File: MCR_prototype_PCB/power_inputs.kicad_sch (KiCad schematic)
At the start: 11 parts, among them J1 Conn_01x20_Pin, U20 LM2596T-5, U21 LM2596T-3.3

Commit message: Add files via upload
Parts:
- C5, C7: footprint (none) -> Capacitor_THT:CP_Radial_D10.0mm_P5.00mm; KiLib_Generator (none) -> capacitor/THT/other
- C6, C8: footprint (none) -> Capacitor_THT:CP_Radial_D8.0mm_P3.50mm; KiLib_Generator (none) -> capacitor/THT/other
- D1, D2: KiLib_Generator (none) -> diode/THT
- J1: footprint (none) -> Connector_PinHeader_2.54mm:PinHeader_1x20_P2.54mm_Horizontal; KiLib_Generator (none) -> connector/pin_header_socket
- L1, L2: footprint (none) -> Inductor_SMD:L_Bourns_SRR1260
- U20, U21: KiLib_Generator (none) -> package/TO_SOT/THT
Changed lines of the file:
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@@
+			)
+		)
+		(property "KiLib_Generator" "diode/THT"
+			(at 125.73 77.47 0)
+			(hide yes)
+			(show_name no)
+			(do_not_autoplace no)
+			(effects
+				(font
+					(size 1.27 1.27)
+				)
 			)
 		)
@@
 			)
 		)
-		(property "Footprint" ""
+		(property "Footprint" "Inductor_SMD:L_Bourns_SRR1260"
 			(at 132.08 73.66 0)
 			(hide yes)
@@
 			)
 		)
+		(property "KiLib_Generator" "diode/THT"
+			(at 124.46 39.37 0)
+			(hide yes)
+			(show_name no)
+			(do_not_autoplace no)
+			(effects
+				(font
+					(size 1.27 1.27)
+				)
+			)
+		)
 		(pin "1"
 		)
@@
 			)
 		)
-		(property "Footprint" ""
+		(property "Footprint" "Capacitor_THT:CP_Radial_D10.0mm_P5.00mm"
 			(at 82.55 71.12 0)
 			(hide yes)
@@
 		)
 		(property "Description" "capacitor, small US symbol"
+			(at 82.55 71.12 0)
+			(hide yes)
+			(show_name no)
+			(do_not_autoplace no)
+			(effects
+				(font
+					(size 1.27 1.27)
+				)
+			)
+		)
+		(property "KiLib_Generator" "capacitor/THT/other"
 			(at 82.55 71.12 0)
 			(hide yes)
@@
 			)
 		)
-		(property "Footprint" ""
+		(property "Footprint" "Inductor_SMD:L_Bourns_SRR1260"
 			(at 130.81 35.56 0)
 			(hide yes)
@@
 			)
 		)
+		(property "KiLib_Generator" "package/TO_SOT/THT"
+			(at 104.14 33.02 0)
+			(hide yes)
+			(show_name no)
+			(do_not_autoplace no)
+			(effects
+				(font
+					(size 1.27 1.27)
+				)
+			)
+		)
 		(pin "5"
 		)
@@
 			)
 		)
-		(property "Footprint" ""
+		(property "Footprint" "Capacitor_THT:CP_Radial_D10.0mm_P5.00mm"
 			(at 82.55 33.02 0)
 			(hide yes)
@@
 		)
 		(property "Description" "capacitor, small US symbol"
+			(at 82.55 33.02 0)
+			(hide yes)
+			(show_name no)
+			(do_not_autoplace no)
+			(effects
+				(font
+					(size 1.27 1.27)
+				)
+			)
+		)
+		(property "KiLib_Generator" "capacitor/THT/other"
 			(at 82.55 33.02 0)
 			(hide yes)
@@
 			)
 		)
+		(property "KiLib_Generator" "package/TO_SOT/THT"
+			(at 104.14 71.12 0)
+			(hide yes)
+			(show_name no)
+			(do_not_autoplace no)
+			(effects
+				(font
+					(size 1.27 1.27)
+				)
+			)
+		)
 		(pin "1"
 		)
@@
 			)
 		)
-		(property "Footprint" ""
+		(property "Footprint" "Connector_PinHeader_2.54mm:PinHeader_1x20_P2.54mm_Horizontal"
 			(at 34.29 50.8 0)
 			(hide yes)
@@
 		)
 		(property "Description" "Generic connector, single row, 01x20, script generated"
+			(at 34.29 50.8 0)
+			(hide yes)
+			(show_name no)
+			(do_not_autoplace no)
+			(effects
+				(font
+					(size 1.27 1.27)
+				)
+			)
+		)
+		(property "KiLib_Generator" "connector/pin_header_socket"
 			(at 34.29 50.8 0)
 			(hide yes)
@@
 			)
 		)
-		(property "Footprint" ""
+		(property "Footprint" "Capacitor_THT:CP_Radial_D8.0mm_P3.50mm"
 			(at 137.16 38.1 0)
 			(hide yes)
@@
 		)
 		(property "Description" "capacitor, small US symbol"
+			(at 137.16 38.1 0)
+			(hide yes)
+			(show_name no)
+			(do_not_autoplace no)
+			(effects
+				(font
+					(size 1.27 1.27)
+				)
+			)
+		)
+		(property "KiLib_Generator" "capacitor/THT/other"
 			(at 137.16 38.1 0)
 			(hide yes)
@@
 			)
 		)
-		(property "Footprint" ""
+		(property "Footprint" "Capacitor_THT:CP_Radial_D8.0mm_P3.50mm"
 			(at 138.43 76.2 0)
 			(hide yes)
@@
 			(at 138.43 76.2 0)
 			(hide yes)
+			(show_name no)
+			(do_not_autoplace no)
+			(effects
+				(font
+					(size 1.27 1.27)
+				)
+			)
+		)
+		(property "KiLib_Generator" "capacitor/THT/other"
+			(at 138.43 76.2 0)
+			(hide yes)

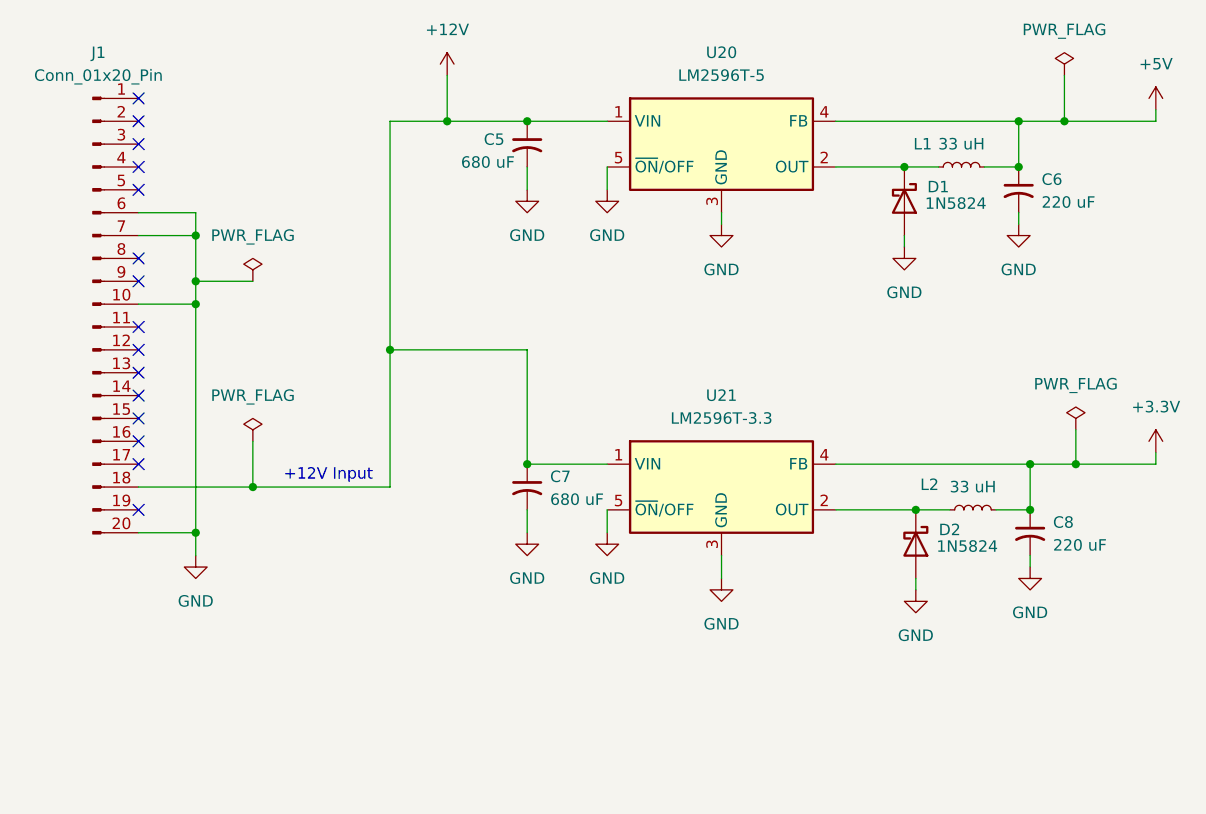
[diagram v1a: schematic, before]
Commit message: Updated 8/22/26
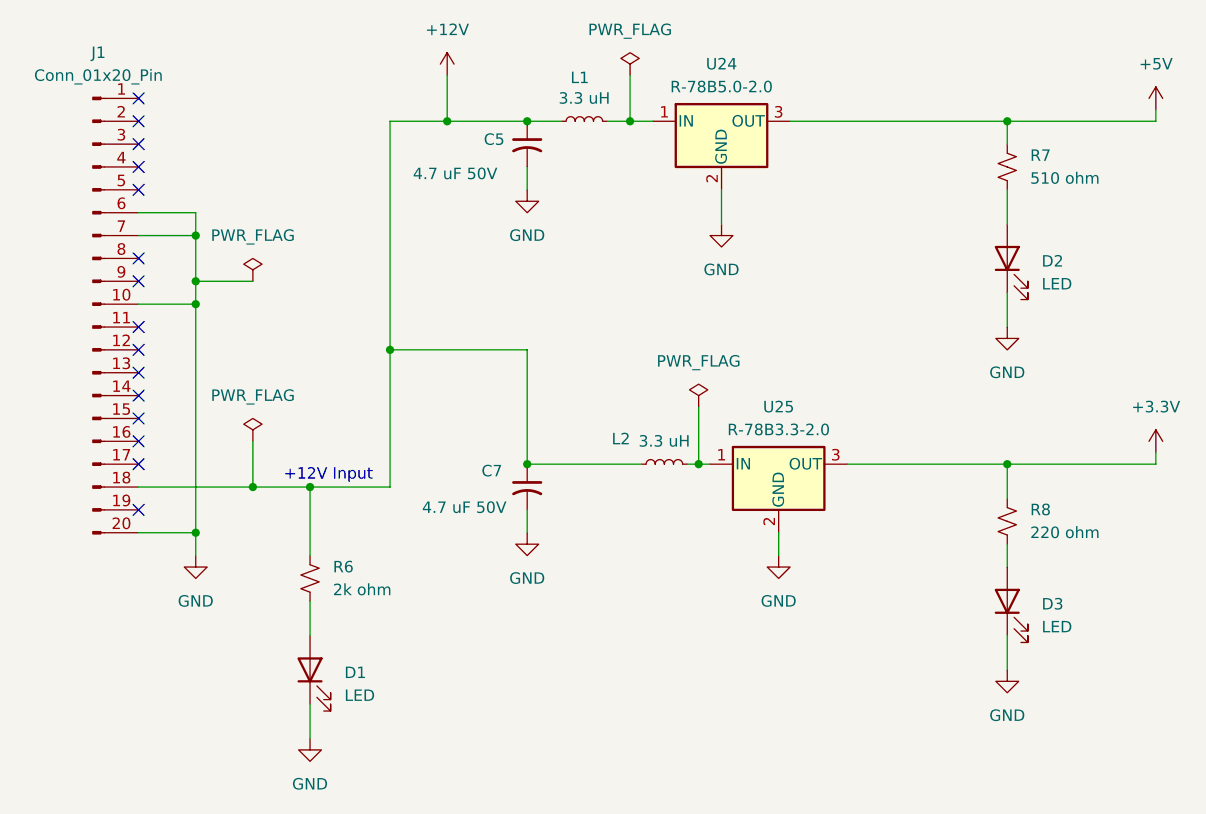
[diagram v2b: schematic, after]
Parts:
- removed C6, C8: 220 uF, Capacitor_THT:CP_Radial_D8.0mm_P3.50mm, symbol Device:C_Small_US
- removed D1, D2: 1N5824, Diode_THT:D_DO-201AD_P15.24mm_Horizontal, symbol Diode:1N5822
- removed U20: LM2596T-5, Package_TO_SOT_THT:TO-220-5_P3.4x3.7mm_StaggerOdd_Lead3.8mm_Vertical, symbol Regulator_Switching:LM2596T-5
- removed U21: LM2596T-3.3, Package_TO_SOT_THT:TO-220-5_P3.4x3.7mm_StaggerOdd_Lead3.8mm_Vertical, symbol Regulator_Switching:LM2596T-3.3
- added D1, D2, D3: LED, LED_SMD:LED_0805_2012Metric_Pad1.15x1.40mm_HandSolder, symbol Device:LED
- added R6: 2k ohm, Resistor_SMD:R_0805_2012Metric_Pad1.20x1.40mm_HandSolder, symbol Device:R_Small_US
- added R7: 510 ohm, Resistor_SMD:R_0805_2012Metric_Pad1.20x1.40mm_HandSolder, symbol Device:R_Small_US
- added R8: 220 ohm, Resistor_SMD:R_0805_2012Metric_Pad1.20x1.40mm_HandSolder, symbol Device:R_Small_US
- added U24: R-78B5.0-2.0, Converter_DCDC:Converter_DCDC_RECOM_R-78B-2.0_THT, symbol Converter_DCDC:R-78B5.0-2.0
- added U25: R-78B3.3-2.0, Converter_DCDC:Converter_DCDC_RECOM_R-78B-2.0_THT, symbol Converter_DCDC:R-78B3.3-2.0
- C5, C7: value 680 uF -> 4.7 uF 50V
- L1, L2: value 33 uH -> 3.3 uH
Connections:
- net +12V: now also L1.1, L2.1, R6.1
- net +3.3V: now also R8.1, U25.3 (OUT); no longer L2.2
- net +5V: now also R7.1, U24.3 (OUT); no longer L1.2
- net GND: now also D1.1 (K), D2.1 (K), D3.1 (K), U24.2 (GND), U25.2 (GND)
- new net: L2.2, U25.1 (IN)
- new net: D1.2 (A), R6.2
- new net: D2.2 (A), R7.2
- new net: D3.2 (A), R8.2
- new net: L1.2, U24.1 (IN)
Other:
- moved on the sheet: L1, L2
